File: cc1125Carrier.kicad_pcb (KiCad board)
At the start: 2 copper layers, 65.9 x 78 mm, 7 parts, among them J1 TFM-110-02-SM-D-A-K-TR, J2 TFM-110-02-SM-D-A-K-TR, J3 Jumper Block, J4 Conn_01x06, U1 YAAJ_WeAct_BlackPill_Part_Lik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

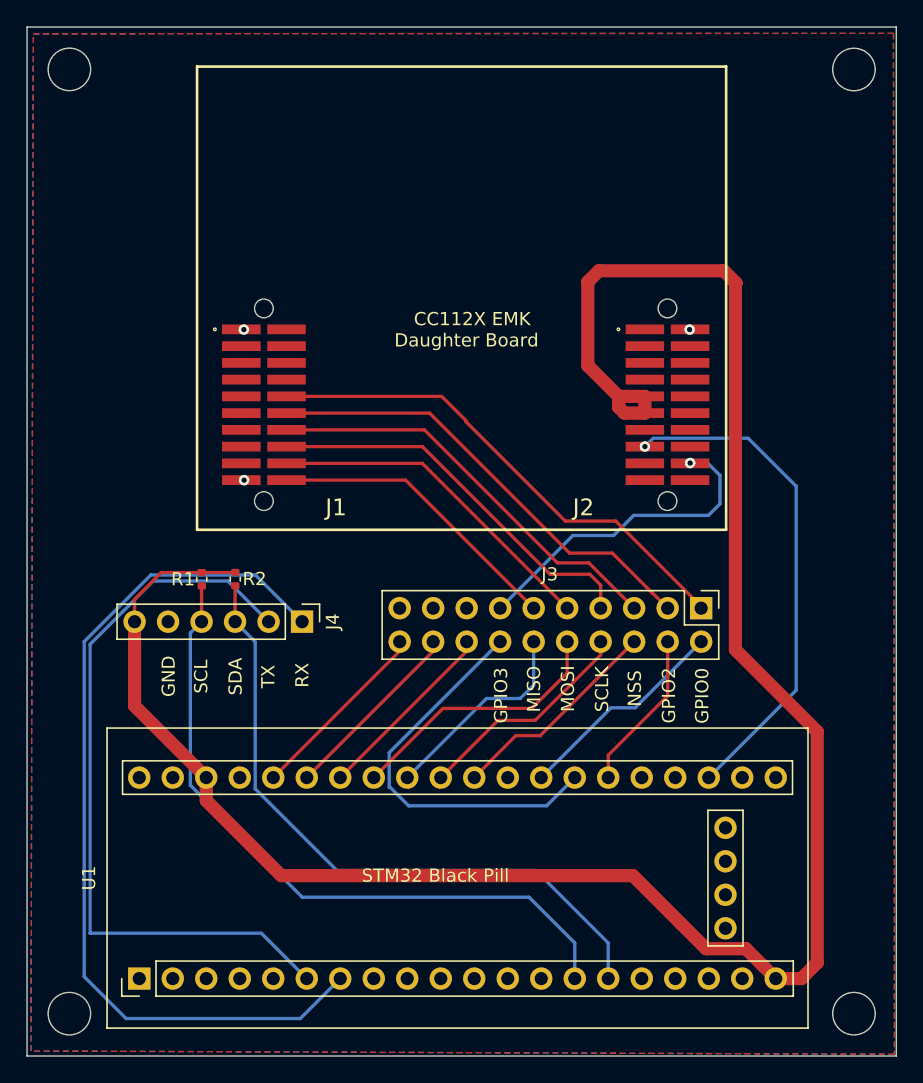
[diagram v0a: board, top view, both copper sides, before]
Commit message: minor board tweaks
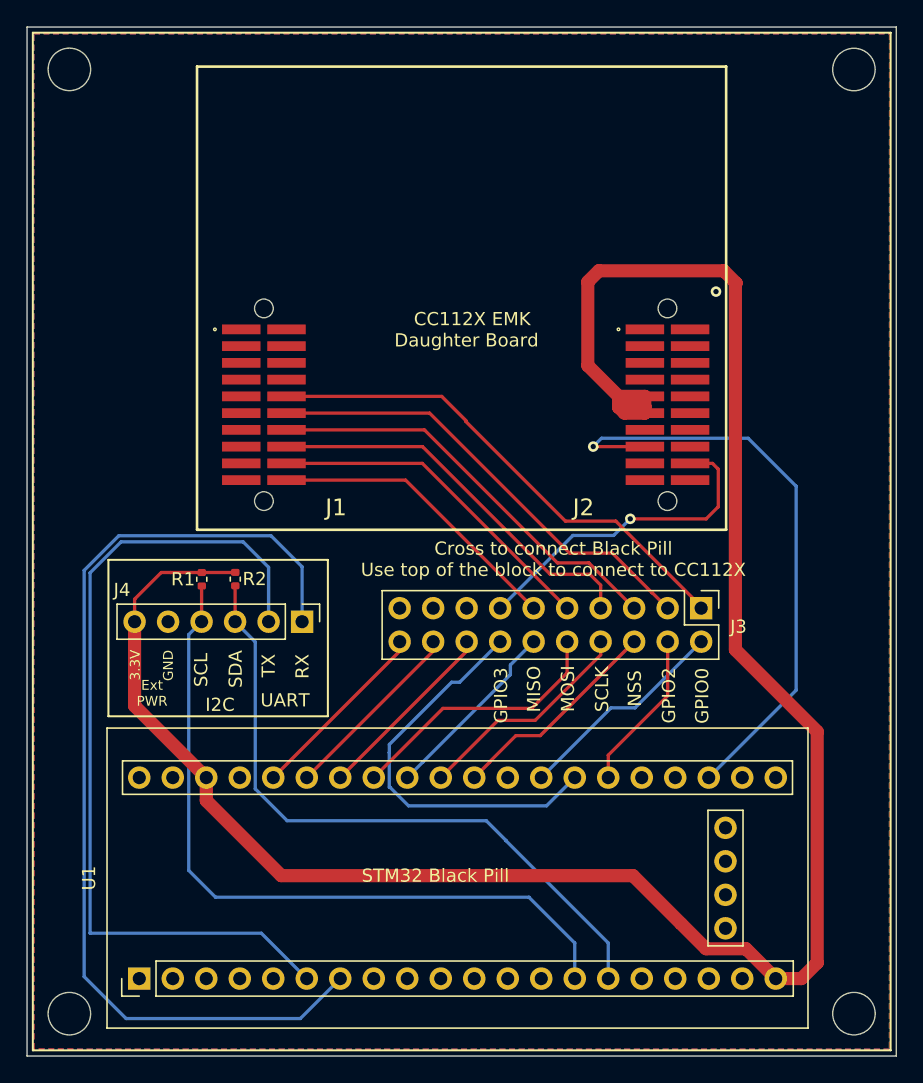
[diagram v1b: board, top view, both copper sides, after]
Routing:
- net RX: track 67.5 -> 75.5 mm
- net TX: track 56.6 -> 64.6 mm
- net NRST: track 38.1 -> 45.9 mm
- net SCL: track 52.3 -> 56.2 mm
- net MCU_VCC: track 160.4 -> 162.4 mm
- net MISO: track 15.8 -> 14.3 mm
- net GND: vias 3 -> 1
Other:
- board text added: "3.3V"
- board text added: "Cross to connect Black Pill Use top of the block to connect to CC112X"
- board text added: "Ext PWR"
- board text added: "I2C"
- board text added: "UART"
